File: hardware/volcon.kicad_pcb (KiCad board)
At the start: 2 copper layers, 112 x 112 mm, 29 parts, among them J1 usb-c_2.0, J2 AVR-ISP-6, J3 4-Pin, Q1 NPN, Q2 NPN, U1 ATmega32U4, Y1 16MHz

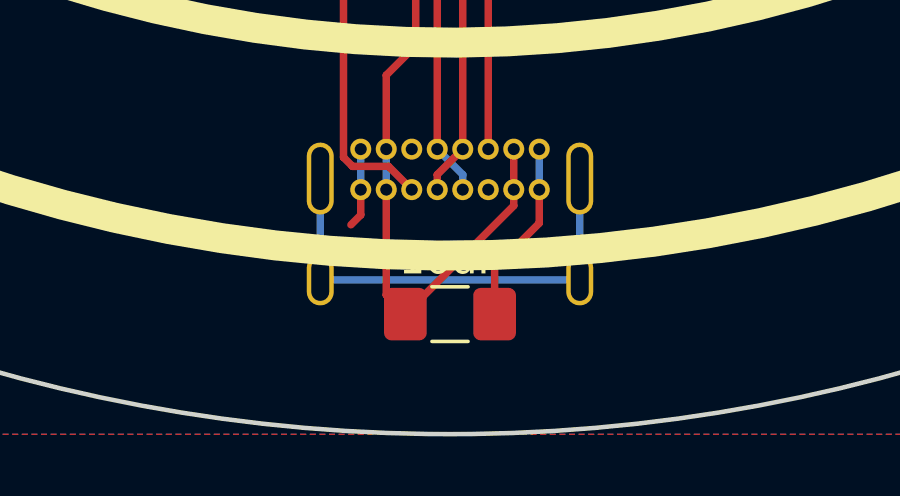
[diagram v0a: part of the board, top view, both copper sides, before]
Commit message: Minor adjustments, clean-up and comments.  Generated schematic pdf for repo.
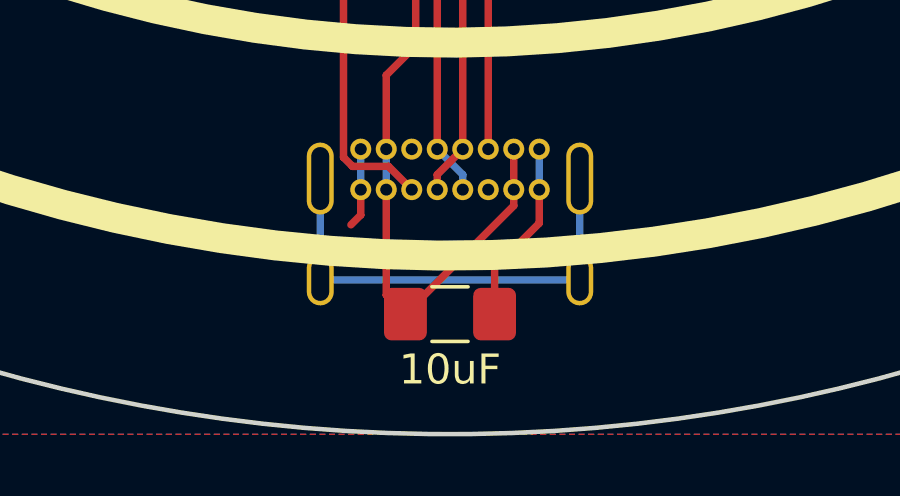
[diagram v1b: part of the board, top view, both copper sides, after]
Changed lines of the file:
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@@
     (pad_to_mask_clearance 0.05)
     (aux_axis_origin 0 0)
-    (visible_elements FFFFFF7F)
+    (visible_elements FEFFFF7F)
     (pcbplotparams
       (layerselection 0x010fc_ffffffff)
@@
       (effects (font (size 1 1) (thickness 0.15)))
     )
-    (fp_text user %R (at 0.3 0) (layer F.Fab)
-      (effects (font (size 1 1) (thickness 0.15)))
-    )
     (fp_circle (center 0 0) (end 2.85 0) (layer Cmts.User) (width 0.15))
     (fp_circle (center 0 0) (end 3.1 0) (layer F.CrtYd) (width 0.05))
+    (fp_text user %R (at 0.3 0) (layer F.Fab)
+      (effects (font (size 1 1) (thickness 0.15)))
+    )
     (pad 1 thru_hole circle (at 0 0) (size 5.7 5.7) (drill 3.2) (layers *.Cu *.Mask))
   )
@@
       (effects (font (size 1 1) (thickness 0.15)))
     )
-    (fp_text user %R (at 0.3 0) (layer F.Fab)
-      (effects (font (size 1 1) (thickness 0.15)))
-    )
     (fp_circle (center 0 0) (end 2.85 0) (layer Cmts.User) (width 0.15))
     (fp_circle (center 0 0) (end 3.1 0) (layer F.CrtYd) (width 0.05))
+    (fp_text user %R (at 0.3 0) (layer F.Fab)
+      (effects (font (size 1 1) (thickness 0.15)))
+    )
     (pad 1 thru_hole circle (at 0 0) (size 5.7 5.7) (drill 3.2) (layers *.Cu *.Mask))
   )
@@
     (fp_text value 22pF (at 0 1.82) (layer F.SilkS)
       (effects (font (size 1 1) (thickness 0.15)))
-    )
-    (fp_text user %R (at 0 0) (layer F.Fab)
-      (effects (font (size 0.8 0.8) (thickness 0.12)))
     )
     (fp_line (start -1.6 0.8) (end -1.6 -0.8) (layer F.Fab) (width 0.1))
@@
     (fp_line (start 2.45 -1.12) (end 2.45 1.12) (layer F.CrtYd) (width 0.05))
     (fp_line (start 2.45 1.12) (end -2.45 1.12) (layer F.CrtYd) (width 0.05))
+    (fp_text user %R (at 0 0) (layer F.Fab)
+      (effects (font (size 0.8 0.8) (thickness 0.12)))
+    )
     (pad 2 smd roundrect (at 1.4875 0) (size 1.425 1.75) (layers F.Cu F.Paste F.Mask) (roundrect_rratio 0.175439)
       (net 1 GND))
@@
       (effects (font (size 1 1) (thickness 0.15)))
     )
-    (fp_text user %R (at 0 0 90) (layer F.Fab)
-      (effects (font (size 0.8 0.8) (thickness 0.12)))
-    )
     (fp_line (start -1.6 0.8) (end -1.6 -0.8) (layer F.Fab) (width 0.1))
     (fp_line (start -1.6 -0.8) (end 1.6 -0.8) (layer F.Fab) (width 0.1))
@@
     (fp_line (start 2.45 -1.12) (end 2.45 1.12) (layer F.CrtYd) (width 0.05))
     (fp_line (start 2.45 1.12) (end -2.45 1.12) (layer F.CrtYd) (width 0.05))
+    (fp_text user %R (at 0 0 90) (layer F.Fab)
+      (effects (font (size 0.8 0.8) (thickness 0.12)))
+    )
     (pad 2 smd roundrect (at 1.4875 0 270) (size 1.425 1.75) (layers F.Cu F.Paste F.Mask) (roundrect_rratio 0.175439)
       (net 1 GND))
@@
       (effects (font (size 1 1) (thickness 0.15)))
     )
-    (fp_text value 10uF (at 0 1.82) (layer F.SilkS)
+    (fp_text value 10uF (at 0 -1.848) (layer F.SilkS)
       (effects (font (size 1 1) (thickness 0.15)))
     )
@@
     (fp_text value LED (at 0.03 -1.966) (layer F.SilkS)
       (effects (font (size 1 1) (thickness 0.15)))
-    )
-    (fp_text user %R (at 0 0) (layer F.Fab)
-      (effects (font (size 0.5 0.5) (thickness 0.05)))
     )
     (fp_line (start -1.8 -1.1) (end 1.8 -1.1) (layer F.CrtYd) (width 0.05))
@@
     (fp_line (start 0.8 -0.8) (end 0.8 0.8) (layer F.Fab) (width 0.1))
     (fp_line (start -0.8 -0.8) (end 0.8 -0.8) (layer F.Fab) (width 0.1))
+    (fp_text user %R (at 0 0) (layer F.Fab)
+      (effects (font (size 0.5 0.5) (thickness 0.05)))
+    )
     (pad 2 smd rect (at 0.88 0 180) (size 1.25 1.6) (layers F.Cu F.Paste F.Mask)
       (net 6 "Net-(D1-Pad2)"))
@@
       (effects (font (size 1 1) (thickness 0.15)))
     )
-    (fp_text user %R (at 0 0 90) (layer F.Fab)
-      (effects (font (size 0.8 0.8) (thickness 0.12)))
-    )
     (fp_line (start 1.91 3.41) (end 1.91 2.15) (layer F.SilkS) (width 0.12))
     (fp_line (start 1.91 -3.41) (end 1.91 -2.15) (layer F.SilkS) (width 0.12))
@@
     (fp_line (start -1.85 3.35) (end 1.85 3.35) (layer F.Fab) (width 0.1))
     (fp_line (start 1.85 -3.35) (end 1.85 3.35) (layer F.Fab) (width 0.1))
+    (fp_text user %R (at 0 0 90) (layer F.Fab)
+      (effects (font (size 0.8 0.8) (thickness 0.12)))
+    )
     (pad 1 smd rect (at -3.15 -2.3 180) (size 2 1.5) (layers F.Cu F.Paste F.Mask)
       (net 23 "Net-(J3-Pad4)"))
@@
       (effects (font (size 1 1) (thickness 0.15)))
     )
-    (fp_text user %R (at 0 0 90) (layer F.Fab)
-      (effects (font (size 0.8 0.8) (thickness 0.12)))
-    )
     (fp_line (start -1.6 0.8) (end -1.6 -0.8) (layer F.Fab) (width 0.1))
     (fp_line (start -1.6 -0.8) (end 1.6 -0.8) (layer F.Fab) (width 0.1))
@@
     (fp_line (start 2.45 -1.12) (end 2.45 1.12) (layer F.CrtYd) (width 0.05))
     (fp_line (start 2.45 1.12) (end -2.45 1.12) (layer F.CrtYd) (width 0.05))
+    (fp_text user %R (at 0 0 90) (layer F.Fab)
+      (effects (font (size 0.8 0.8) (thickness 0.12)))
+    )
     (pad 2 smd roundrect (at 1.4875 0 270) (size 1.425 1.75) (layers F.Cu F.Paste F.Mask) (roundrect_rratio 0.175439)
       (net 19 !RESET))
@@
       (effects (font (size 1 1) (thickness 0.15)))
     )
-    (fp_text user %R (at 0 0 90) (layer F.Fab)
-      (effects (font (size 0.8 0.8) (thickness 0.12)))
-    )
     (fp_line (start -1.6 0.8) (end -1.6 -0.8) (layer F.Fab) (width 0.1))
     (fp_line (start -1.6 -0.8) (end 1.6 -0.8) (layer F.Fab) (width 0.1))
@@
     (fp_line (start 2.45 -1.12) (end 2.45 1.12) (layer F.CrtYd) (width 0.05))
     (fp_line (start 2.45 1.12) (end -2.45 1.12) (layer F.CrtYd) (width 0.05))
+    (fp_text user %R (at 0 0 90) (layer F.Fab)
+      (effects (font (size 0.8 0.8) (thickness 0.12)))
+    )
     (pad 2 smd roundrect (at 1.4875 0 270) (size 1.425 1.75) (layers F.Cu F.Paste F.Mask) (roundrect_rratio 0.175439)
       (net 15 "Net-(J1-PadB5)"))
@@
       (effects (font (size 1 1) (thickness 0.15)))
     )
-    (fp_text user %R (at 0 0 90) (layer F.Fab)
-      (effects (font (size 0.8 0.8) (thickness 0.12)))
-    )
     (fp_line (start -1.6 0.8) (end -1.6 -0.8) (layer F.Fab) (width 0.1))
     (fp_line (start -1.6 -0.8) (end 1.6 -0.8) (layer F.Fab) (width 0.1))
@@
     (fp_line (start 2.45 -1.12) (end 2.45 1.12) (layer F.CrtYd) (width 0.05))
     (fp_line (start 2.45 1.12) (end -2.45 1.12) (layer F.CrtYd) (width 0.05))
+    (fp_text user %R (at 0 0 90) (layer F.Fab)
+      (effects (font (size 0.8 0.8) (thickness 0.12)))
+    )
     (pad 2 smd roundrect (at 1.4875 0 270) (size 1.425 1.75) (layers F.Cu F.Paste F.Mask) (roundrect_rratio 0.175439)
       (net 1 GND))
@@
       (effects (font (size 1 1) (thickness 0.15)))
     )
-    (fp_text user %R (at 0 0) (layer F.Fab)
-      (effects (font (size 0.8 0.8) (thickness 0.12)))
-    )
     (fp_line (start -1.6 0.8) (end -1.6 -0.8) (layer F.Fab) (width 0.1))
     (fp_line (start -1.6 -0.8) (end 1.6 -0.8) (layer F.Fab) (width 0.1))
@@
     (fp_line (start 2.45 -1.12) (end 2.45 1.12) (layer F.CrtYd) (width 0.05))
     (fp_line (start 2.45 1.12) (end -2.45 1.12) (layer F.CrtYd) (width 0.05))
+    (fp_text user %R (at 0 0) (layer F.Fab)
+      (effects (font (size 0.8 0.8) (thickness 0.12)))
+    )
     (pad 2 smd roundrect (at 1.4875 0 180) (size 1.425 1.75) (layers F.Cu F.Paste F.Mask) (roundrect_rratio 0.175439)
       (net 9 "Net-(D2-Pad2)"))
